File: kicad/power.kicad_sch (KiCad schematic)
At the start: 18 parts, among them T1 475uH, U22 SN6505BDBV, U23 TPS7A39

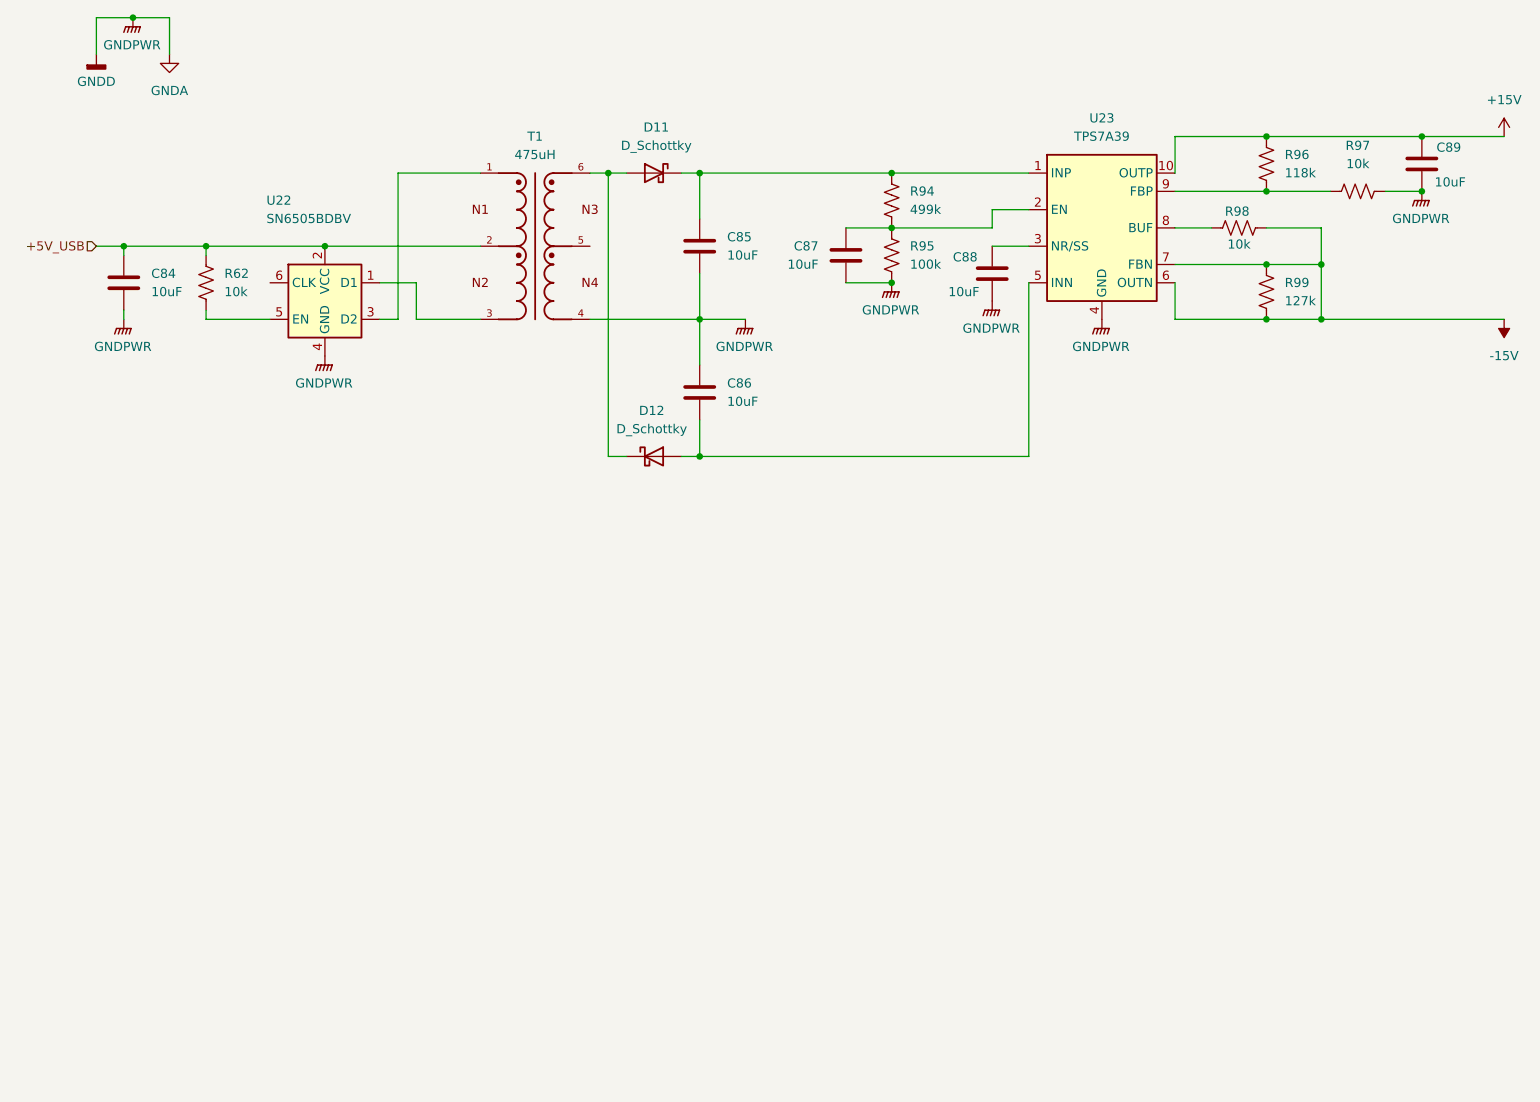
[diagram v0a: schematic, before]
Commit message: power supplies
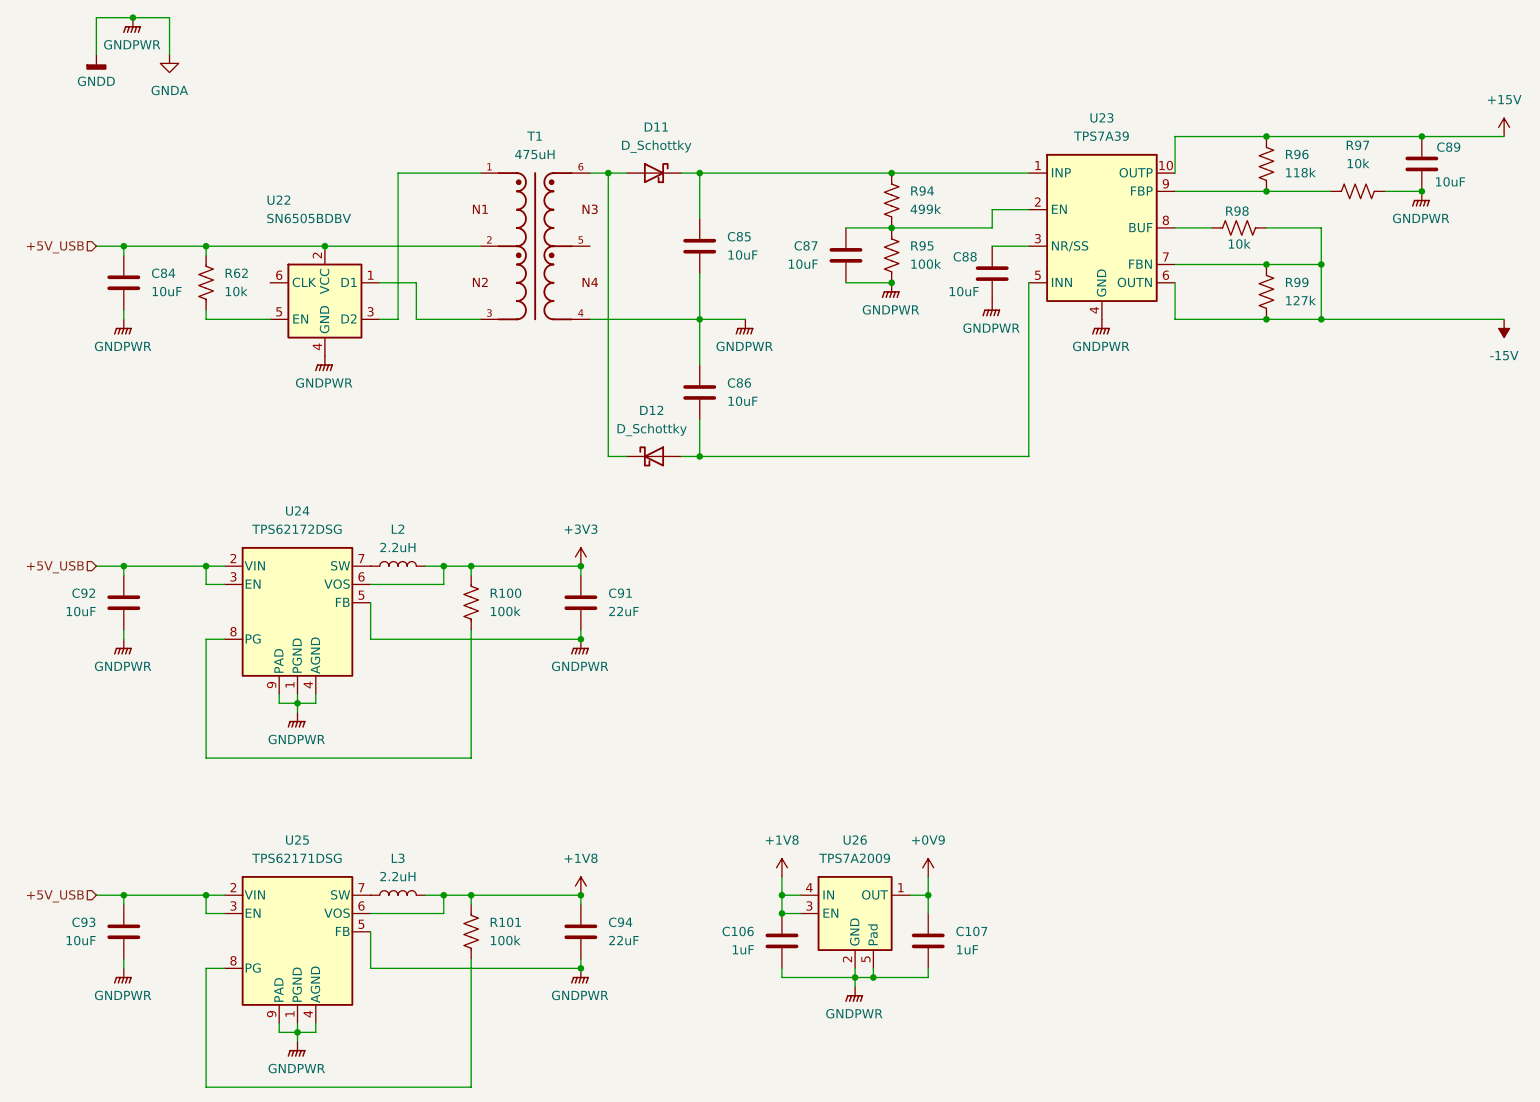
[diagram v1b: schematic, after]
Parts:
- added C106, C107: 1uF, symbol Device:C
- added C91, C94: 22uF, symbol Device:C
- added C92, C93: 10uF, symbol Device:C
- added L2, L3: 2.2uH, symbol Device:L
- added R100, R101: 100k, symbol Device:R_US
- added U24: TPS62172DSG, Package_SON:WSON-8-1EP_2x2mm_P0.5mm_EP0.9x1.6mm_ThermalVias, symbol Regulator_Switching:TPS62172DSG
- added U25: TPS62171DSG, Package_SON:WSON-8-1EP_2x2mm_P0.5mm_EP0.9x1.6mm_ThermalVias, symbol Regulator_Switching:TPS62171DSG
- added U26: TPS7A2009, Package_SON:Texas_X2SON-4_1x1mm_P0.65mm, symbol Regulator_Linear:TPS7A20xxxDQN
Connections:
- net +5V_USB: now also C92.1, C93.1, U24.2 (VIN), U24.3 (EN), U25.2 (VIN), U25.3 (EN)
- net GNDA: now also C106.2, C107.2, C91.2, C92.2, C93.2, C94.2, U24.1 (PGND), U24.4 (AGND), U24.5 (FB), U24.9 (PAD), U25.1 (PGND), U25.4 (AGND), U25.5 (FB), U25.9 (PAD), U26.2 (GND), U26.5 (Pad)
- new net: L3.1, U25.7 (SW)
- new net: R101.2, U25.8 (PG)
- new net: R100.2, U24.8 (PG)
- new net: L2.1, U24.7 (SW)
- new net +0V9: C107.1, U26.1 (OUT)
- new net +1V8: C106.1, C94.1, L3.2, R101.1, U25.6 (VOS), U26.3 (EN), U26.4 (IN)
- new net +3V3: C91.1, L2.2, R100.1, U24.6 (VOS)
